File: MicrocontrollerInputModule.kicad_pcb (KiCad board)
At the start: 2 copper layers, 31 x 111.4 mm, 370 parts, among them J2 FH34SRJ-12S-0.5SH_50_, SW1 KXT3, SW2 KXT3, U1 W25Q16JVUXIQ, U2 RP2040, U3 74AHC125BQ_115, U4 74AHC125BQ_115, Y1 12.000MHz

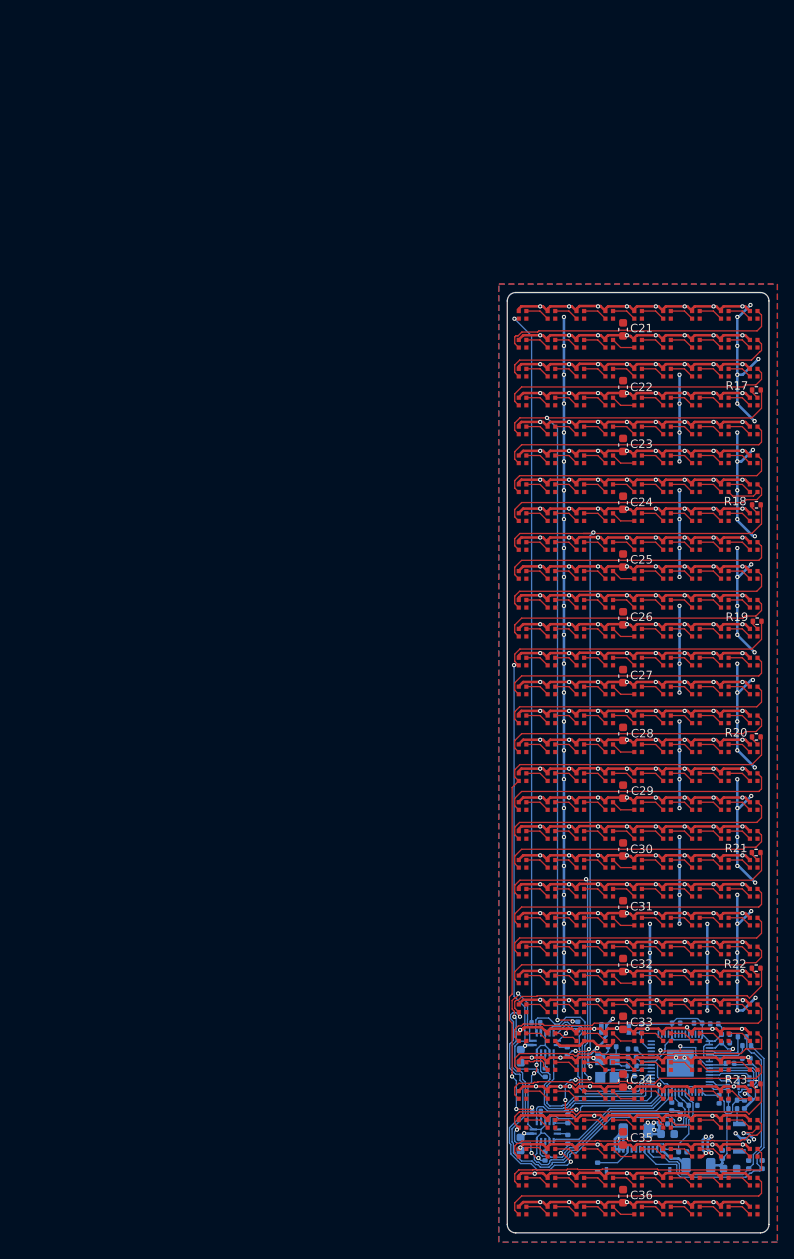
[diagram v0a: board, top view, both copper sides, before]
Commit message: PCB Assembly and Production Files
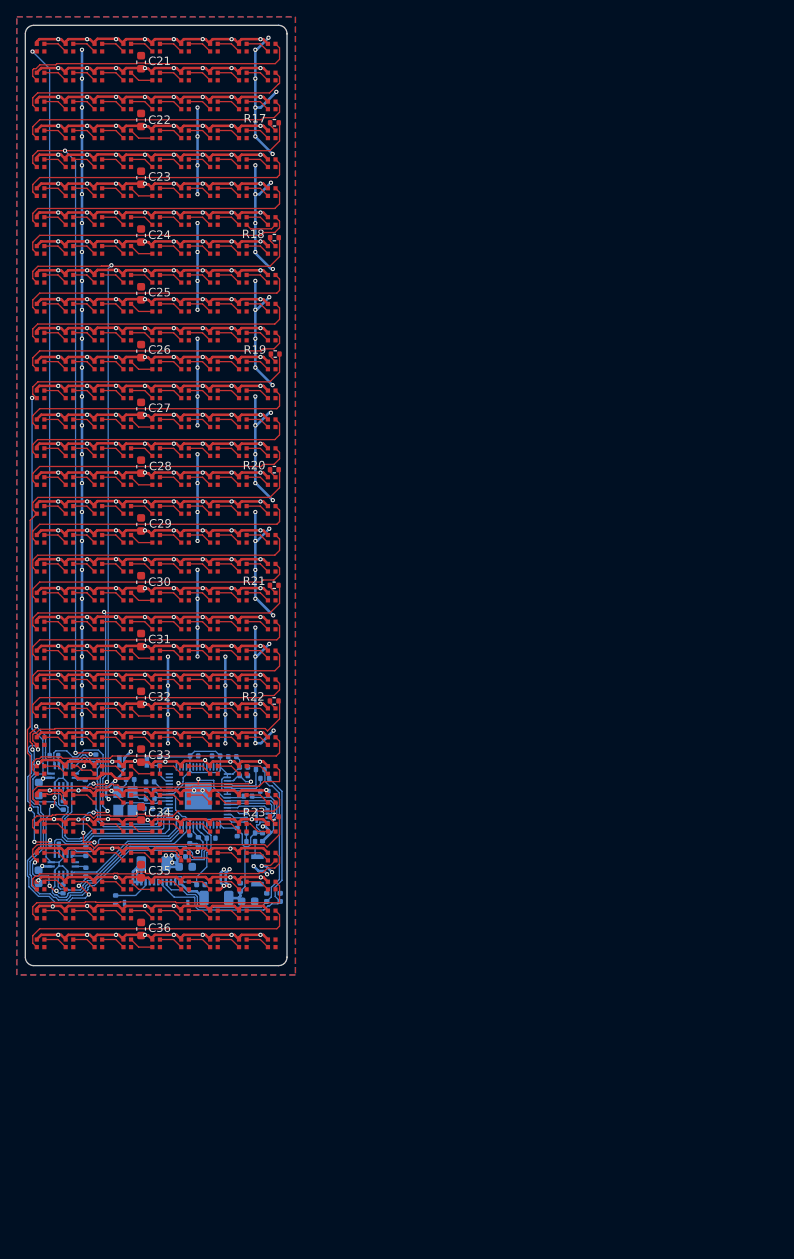
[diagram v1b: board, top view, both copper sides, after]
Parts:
- moved N139 65.3 mm to (42.7, 72.0)
- moved N148 65.3 mm to (42.7, 75.5)
- moved N274 65.3 mm to (42.7, 123.4)
- moved N283 65.3 mm to (42.7, 126.8)
- moved R6 65.3 mm to (58.4, 106.2)
- moved U1 65.3 mm to (58.0, 111.7)
- moved C1 65.3 mm to (45.2, 110.9)
- moved C12 65.3 mm to (50.1, 114.5)
- moved C18 65.3 mm to (32.2, 118.9)
- moved C6 65.3 mm to (56.5, 107.0)
- moved C7 65.3 mm to (55.1, 104.7)
- moved C8 65.3 mm to (56.5, 105.9)
- moved G*** 65.3 mm to (44.3, 97.7)
- moved G*** 65.3 mm to (41.6, 97.8)
- moved G*** 65.3 mm to (38.8, 97.8)
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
